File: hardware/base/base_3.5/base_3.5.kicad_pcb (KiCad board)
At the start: 2 copper layers, 69.7 x 17 mm, 8 parts, among them IC1 single_pad, IC2 single_pad, J1 conn_2x2

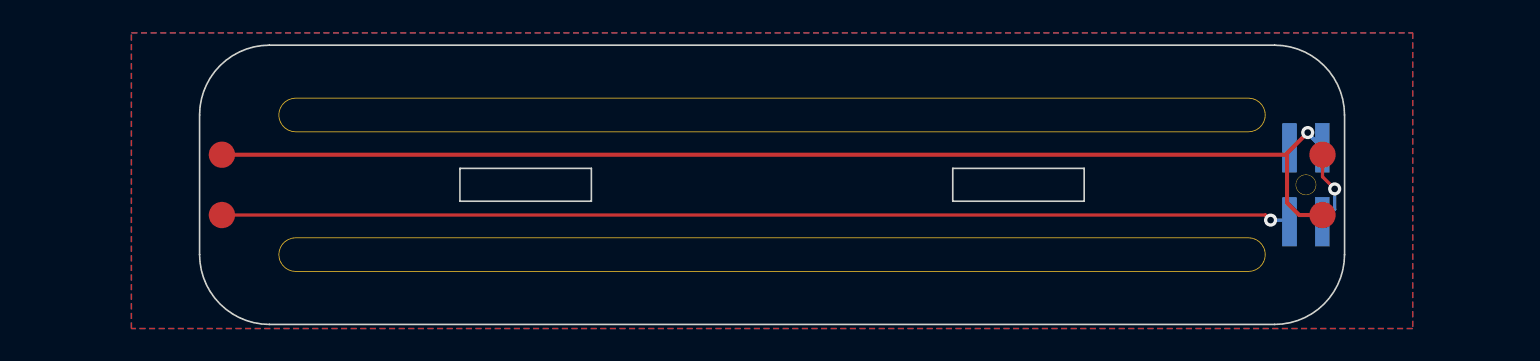
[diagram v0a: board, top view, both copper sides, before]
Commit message: 3.5" PCB layout
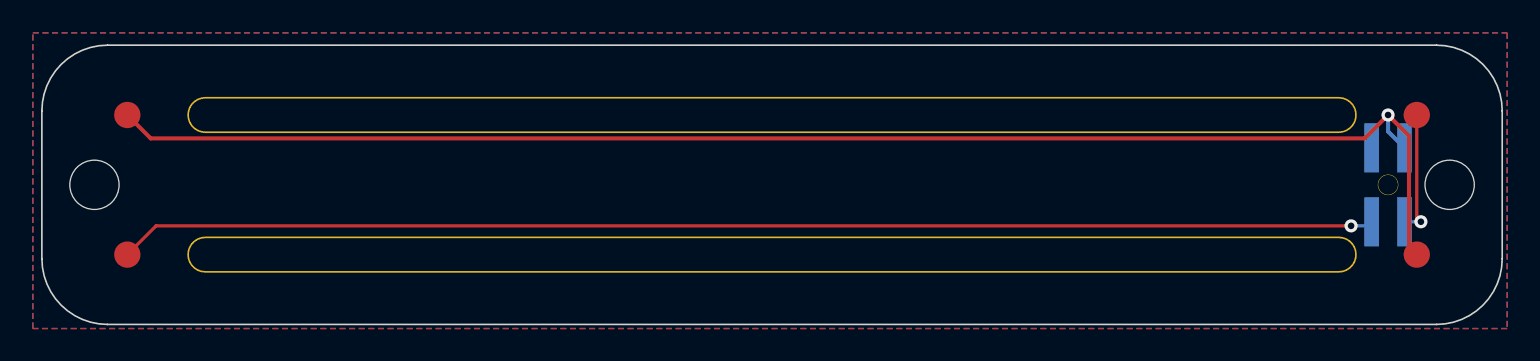
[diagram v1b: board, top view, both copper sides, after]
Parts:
- added H1: MountingHole, cycfi_library:hole_3mm, F.Cu at (166.2, 55.2)
- added H2: MountingHole, cycfi_library:hole_3mm, F.Cu at (83.8, 55.2)
- H5, H6: footprint xr_spectra_library:rail_slot_3.3 -> xr_spectra_library:rail_slot_3.5
- moved IC1 6.25 mm to (85.8, 51.0)
- moved OC2 6.24 mm to (85.8, 59.5)
- moved OC1 6.23 mm to (164.2, 51.0)
- moved IC2 6.23 mm to (164.2, 59.5)
- moved J1 5.00 mm to (162.5, 55.2)
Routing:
- net inner_coil: track 73.4 -> 89.6 mm
- net /out-: track 65.2 -> 76.6 mm
- net /out+: track 4.70 -> 7.60 mm
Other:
- board size 69.7 x 17 mm -> 88.9 x 17 mm
